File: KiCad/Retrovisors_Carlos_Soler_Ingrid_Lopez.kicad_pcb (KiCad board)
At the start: 2 copper layers, 143.5 x 100.8 mm, 127 parts, among them IC1 PIC24H, J1 Conn_01x02, J11 Conn_01x02, J12 Conn_01x02, J14 Conn_01x02_Pin, J2 DE9_Plug_MountingHoles, J3 DE9_Plug_MountingHoles, J3-4 Conn_01x02, J4 Conn_01x03, J5 Conn_01x02, J7 Conn_01x05, J7-8 Conn_01x02, J9 Conn_01x02, K1 G6E, K10 G6E, K2 G6E, K3 G6E, K4 G6E, K5 G6E, K6 G6E, K7 G6E, K8 G6E, K9 G6E, Q1 NMOS, Q10 NMOS, Q11 IRLZ44N, Q12 IRLZ44N, Q2 NMOS, Q3 NMOS, Q4 NMOS, Q5 NMOS, Q6 NMOS, Q7 NMOS, Q8 NMOS, Q9 NMOS, SW1 SW_DP3T, SW2 SW_DP3T, SW3 SW_DP3T, SW4 OP/CL, SW7 OP/CL, U1 TSR0.5-2450, U2 MCP2551-I-SN, U3 PCF8574P, U4 type="X" model="OPAMP" lib="", U5 type="X" model="OPAMP" lib="", U6 LM1117DT-3.3, Y1 Crystal

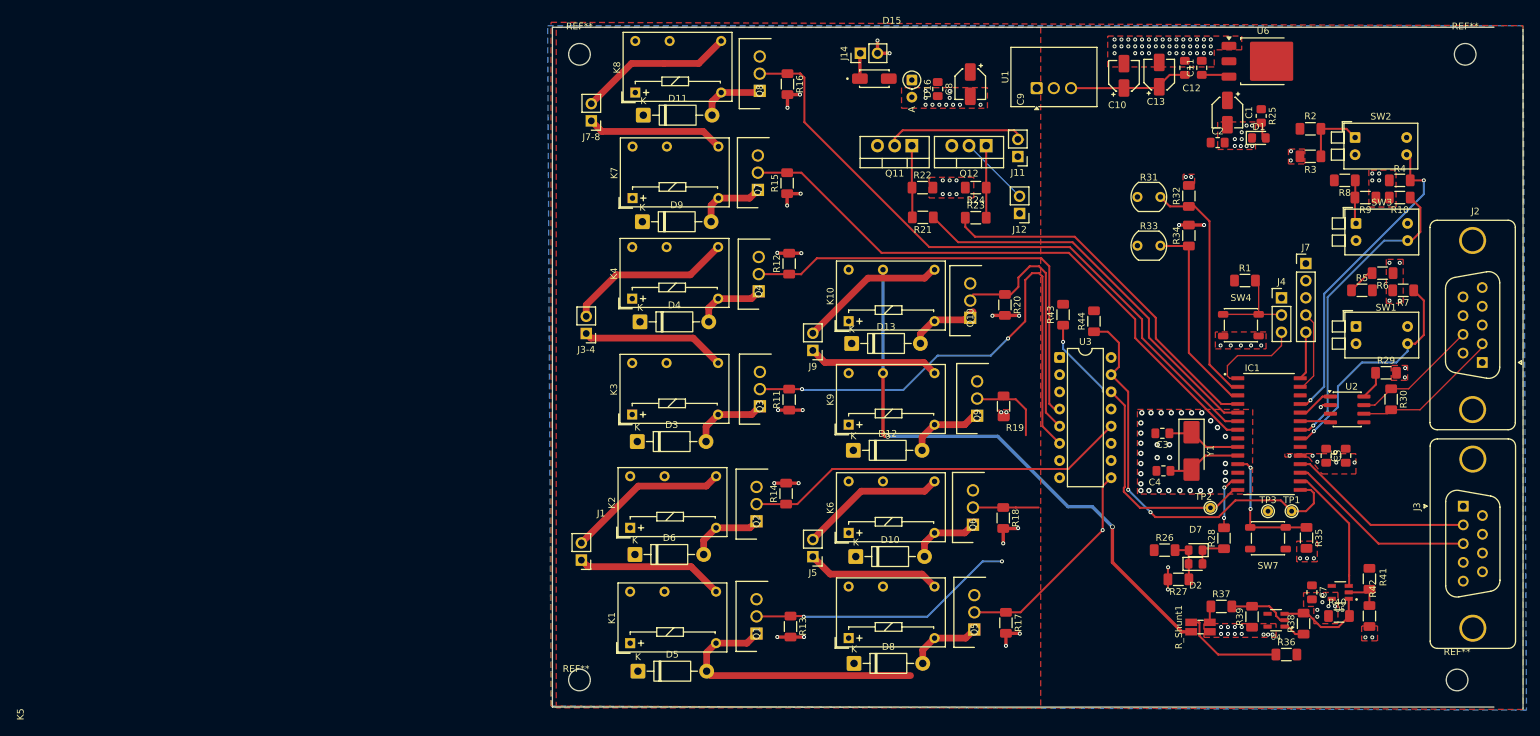
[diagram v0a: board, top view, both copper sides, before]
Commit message: pcb definitiva
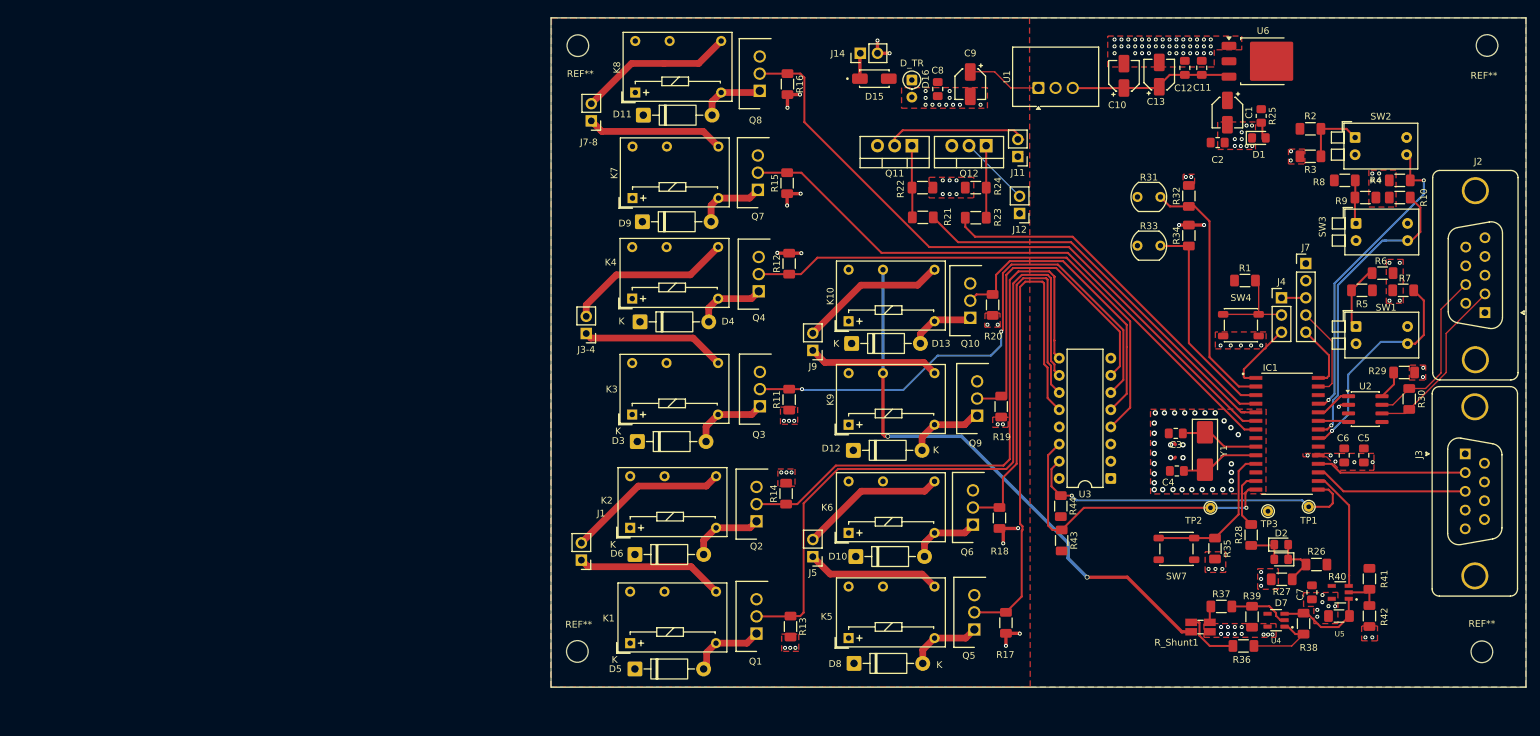
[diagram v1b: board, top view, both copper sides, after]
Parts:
- moved R43 33.4 mm to (126.3, 125.4), turned to -90 degrees
- moved R44 27.8 mm to (126.2, 120.3), turned to -90 degrees
- moved R26 22.5 mm to (164.0, 128.9), turned to 180 degrees
- moved U3 19.4 mm to (133.6, 116.2), turned to 180 degrees
- moved R27 15.3 mm to (158.8, 131.1)
- moved R35 13.6 mm to (149.0, 126.6)
- moved SW7 13.6 mm to (143.3, 126.6)
- moved D2 12.7 mm to (158.8, 126.0), turned to 0 degrees
- moved D7 12.7 mm to (158.8, 128.2), turned to 180 degrees
- moved J3 7.74 mm to (186.0, 112.6)
- moved J2 7.38 mm to (188.9, 91.7)
- moved R36 6.48 mm to (153.2, 141.0)
- moved REF** 5.55 mm to (188.4, 141.8)
- moved REF** 4.23 mm to (54.7, 141.8)
- moved R28 4.04 mm to (154.3, 124.6)
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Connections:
- net /Digital/osc1 renamed /Digital/OSC1
- net /Digital/osc2 renamed /Digital/OSC2
- net Net-(D1-A) renamed /Alimentació/LD_V
- net Net-(D10-A) renamed /Potencia/Vdrain6
- net Net-(D2-A) renamed /Alimentació/ALD2
- net Net-(D2-K) renamed /Alimentació/ALD1
- net Net-(IC1-RA0/AN0) renamed /Digital/AL1
- net Net-(IC1-RA1/AN1) renamed /Digital/AL2
- net Net-(IC1-RC0/T1OSO/T13CKI) renamed /Digital/SP
- net Net-(IC1-RC3/SCK/SCL) renamed /Digital/SCL
- net Net-(IC1-RC4/SDI/SDA) renamed /Digital/SDA
- net Net-(J4-Pin_1) renamed /Digital/ConMu
- net Net-(R2-Pad1) renamed /Digital/LM_BO
- net Net-(R36-Pad1) renamed /Potencia/RSH2
- net Net-(R37-Pad1) renamed /Potencia/RSH3
- net Net-(R5-Pad1) renamed /Digital/RM_BO
- net Net-(R8-Pad1) renamed /Digital/SE_BO
- net Net-(U1-Vout) renamed /Alimentació/V_Buck
- net Net-(U2-Rs) renamed /Digital/RS
- net Net-(U4-+) renamed /Potencia/O1V+
- net Net-(U4--) renamed /Potencia/O1V-
- net Net-(U5-+) renamed /Potencia/O2V+
- net Net-(U5--) renamed /Potencia/O2V-
- U3 pad 12: DLX_D -> DRX_U
- U3 pad 9: DRX_U -> DLX_D
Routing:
- net DLX_U: track 39.9 -> 104.6 mm, vias 2 -> 0
- net DRX_D: track 9.72 -> 60.9 mm
- net DRX_U: track 32.3 -> 77.5 mm, vias 1 -> 0
- net DM_O: track 12.3 -> 50.1 mm
- net /Potencia/Vdrain1: track 41.7 -> 11.3 mm
- net DLX_D: track 57.2 -> 86.5 mm
- net GND: track 48.0 -> 29.5 mm, vias 172 -> 177
- net /Digital/SDA: track 62.7 -> 51.0 mm, vias 2 -> 1
- net VBAT_PROT: track 0.18 -> 11.3 mm
- net DLY_D: track 65.9 -> 76.6 mm
- net /Potencia/O1V+: track 3.27 -> 11.3 mm
- net DM_C: track 37.2 -> 44.2 mm
- net /Potencia/RSH2: track 15.6 -> 8.75 mm
- net /Digital/CAN+: track 19.0 -> 25.3 mm
- net /Digital/RM_BO: track 4.35 -> 9.94 mm
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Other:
- board size 143.5 x 100.8 mm -> 144.1 x 99 mm
